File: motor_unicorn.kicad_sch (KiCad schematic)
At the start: 18 parts, among them J10 Conn_01x06_Pin, J5 Conn_01x03_Socket, J6 Conn_01x03_Socket, J7 Conn_01x06_Pin, J8 Conn_01x06_Pin, J9 Conn_01x06_Pin

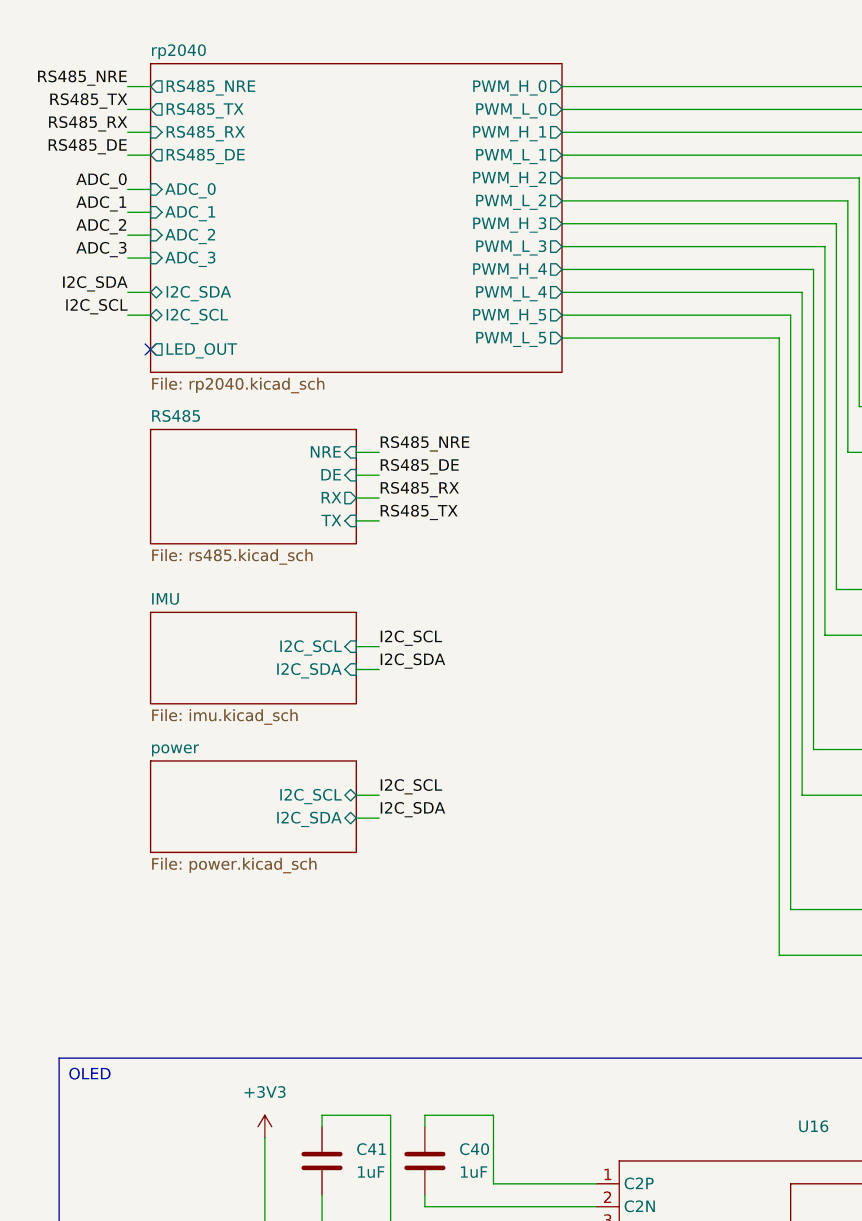
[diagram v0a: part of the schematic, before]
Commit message: more connections
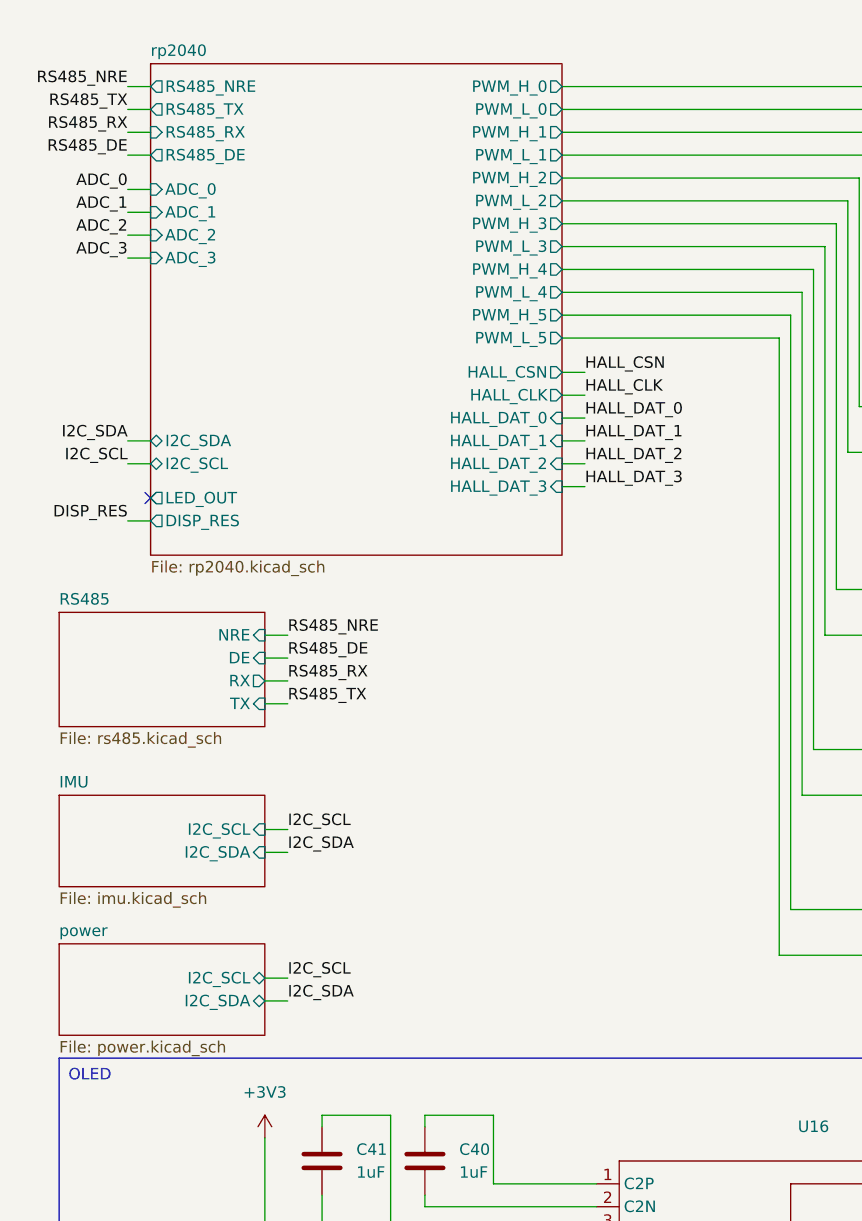
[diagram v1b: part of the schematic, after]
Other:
- sheet rp2040 ports: added DISP_RES, HALL_CLK, HALL_CSN, HALL_DAT_0, HALL_DAT_1, HALL_DAT_2, HALL_DAT_3; removed none
